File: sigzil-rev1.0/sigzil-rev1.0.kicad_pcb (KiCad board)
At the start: 2 copper layers, 172 x 129.5 mm, 81 parts, among them SW1 Keyswitch, SW10 Keyswitch, SW11 Keyswitch, SW12 Keyswitch, SW13 Keyswitch, SW14 Keyswitch, SW15 Keyswitch, SW16 Keyswitch, SW17 Keyswitch, SW18 Keyswitch, SW19 Keyswitch, SW2 Keyswitch, SW20 Keyswitch, SW21 Keyswitch, SW22 Keyswitch, SW23 Keyswitch, SW24 Keyswitch, SW25 Keyswitch, SW26 Keyswitch, SW27 Keyswitch, SW28 Keyswitch, SW29 Keyswitch, SW3 Keyswitch, SW30 Keyswitch, SW31 Keyswitch, SW32 Keyswitch, SW33 Keyswitch, SW34 Keyswitch, SW35 Keyswitch, SW4 Keyswitch, SW5 Keyswitch, SW6 Keyswitch, SW7 Keyswitch, SW8 Keyswitch, SW9 Keyswitch, U1 Arduino_Pro_Micro

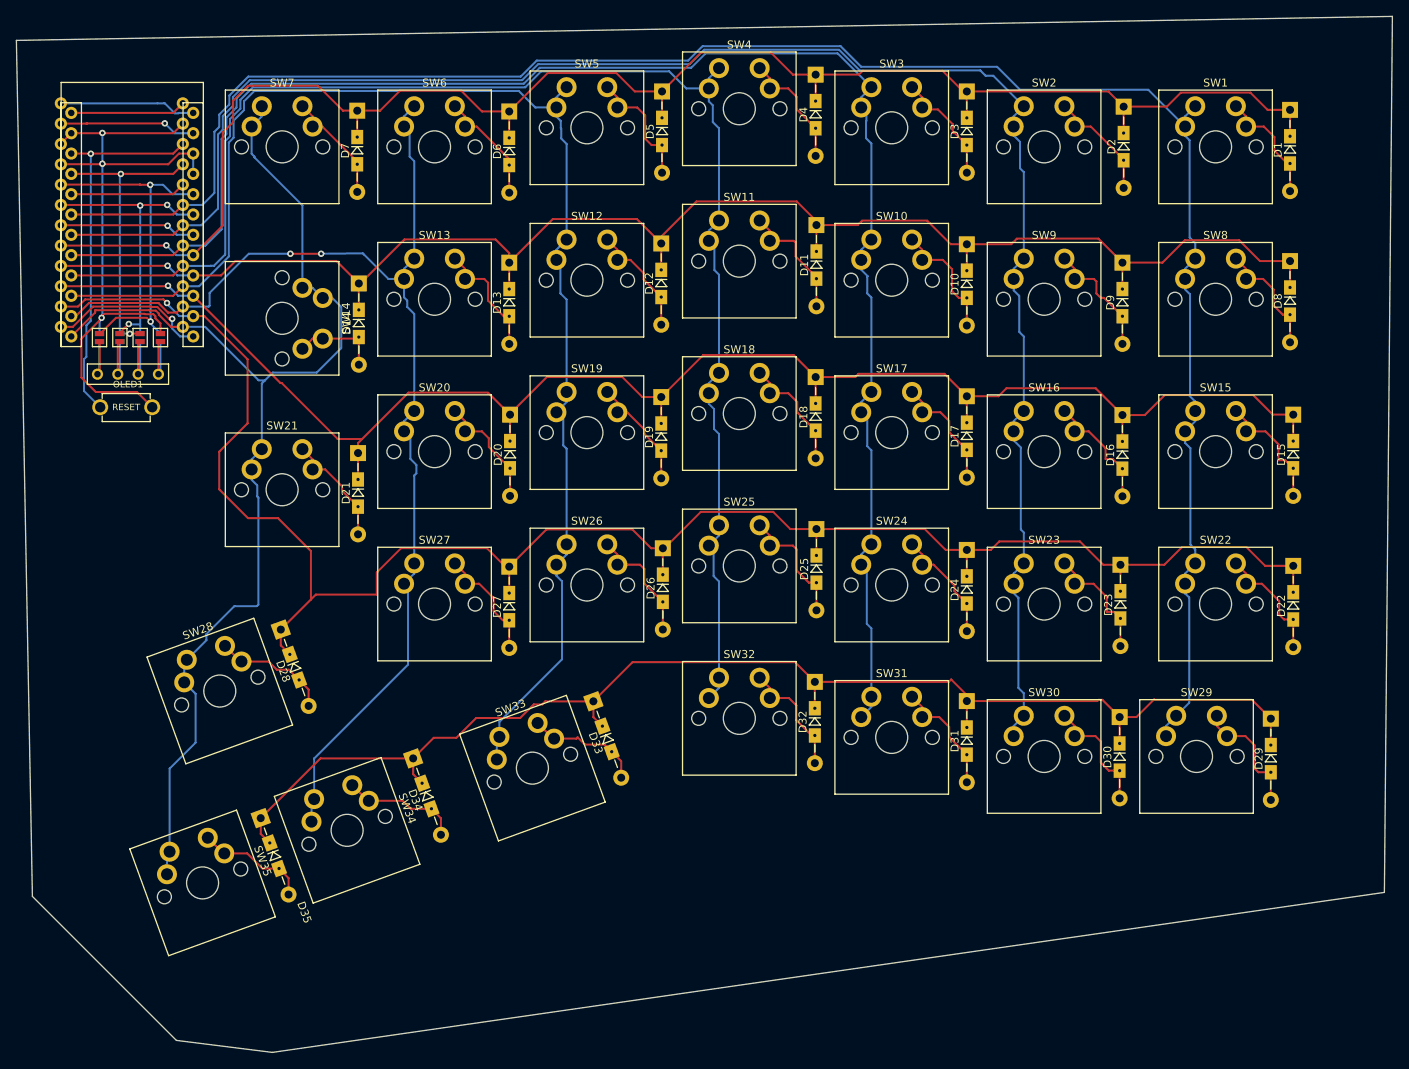
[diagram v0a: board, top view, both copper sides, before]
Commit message: WIP WIP
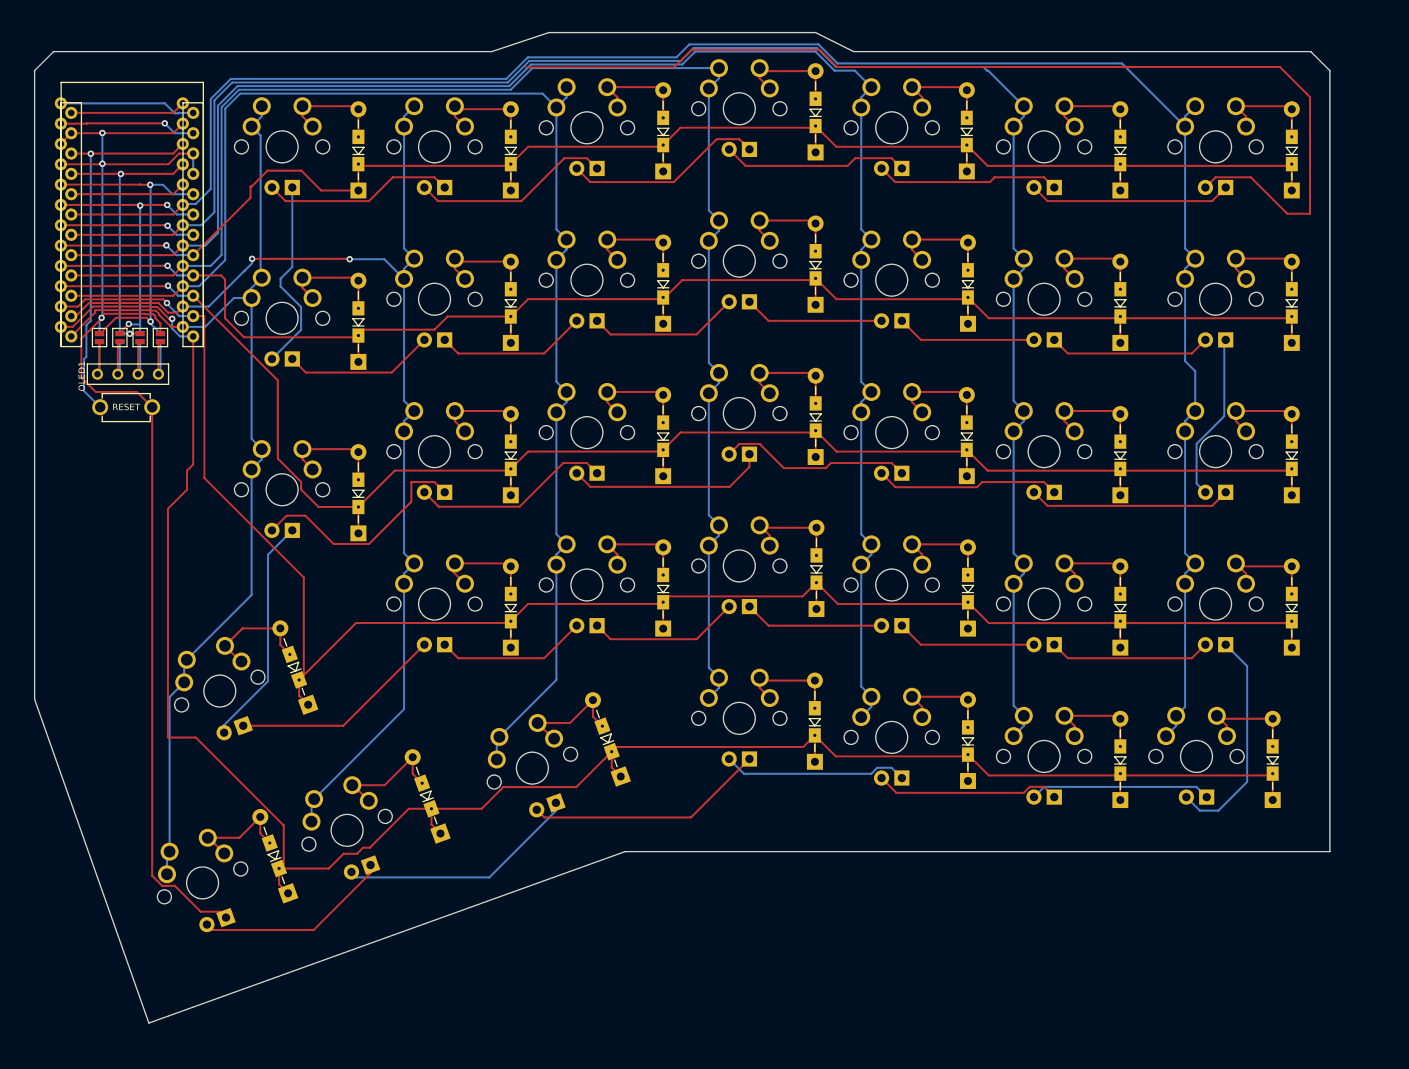
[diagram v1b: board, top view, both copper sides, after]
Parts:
- D1, D10, D11, D12, D13, D14, D15, D16, D17, D18, D19, D2, D20, D21, D22, D23, D24, D25, D26, D27, D28, D29, D3, D30, D31, D32, D33, D34, D35, D4, D5, D6, D7, D8, D9: moved to B.Cu
- SW1, SW15, SW22, SW33, SW8: footprint Sigzil:MX_PCB_1.25u -> Sigzil:MXOnly_Led_1.25u
- SW10, SW11, SW12, SW13, SW16, SW17, SW18, SW19, SW2, SW20, SW21, SW23, SW24, SW25, SW26, SW27, SW28, SW29, SW3, SW30, SW31, SW32, SW4, SW5, SW6, SW7, SW9: footprint Sigzil:MX_PCB_1.00u -> Sigzil:MXOnly_Led_1.00u
- SW14: footprint Sigzil:MX_PCB_1.25u -> Sigzil:MXOnly_Led_1.25u_90deg
- SW34, SW35: footprint Sigzil:MX_PCB_1.25u_90deg -> Sigzil:MXOnly_Led_1.25u_90deg
- moved D2 0.63 mm to (190.3, 54.4), turned to 90 degrees
- moved D30 0.38 mm to (190.3, 130.6), turned to 90 degrees
- moved D23 0.36 mm to (190.3, 111.6), turned to 90 degrees
- moved D8 0.32 mm to (211.8, 73.5), turned to 90 degrees
- moved D29 0.29 mm to (209.4, 130.6), turned to 90 degrees
- moved D22 0.29 mm to (211.8, 111.6), turned to 90 degrees
- moved D4 0.28 mm to (152.2, 49.7), turned to 90 degrees
- moved D19 0.27 mm to (133.2, 90.2), turned to 90 degrees
- moved D9 0.26 mm to (190.3, 73.5), turned to 90 degrees
- moved D16 0.26 mm to (190.3, 92.5), turned to 90 degrees
- moved D12 0.25 mm to (133.2, 71.1), turned to 90 degrees
- moved D27 0.23 mm to (114.1, 111.6), turned to 90 degrees
- moved D1 0.23 mm to (211.8, 54.4), turned to 90 degrees
- moved D6 0.23 mm to (114.1, 54.4), turned to 90 degrees
- moved D24 0.22 mm to (171.3, 109.2), turned to 90 degrees
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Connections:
- U1 pad 7: unconnected-(U1-4/PD4-Pad7) -> BACKLIGHT
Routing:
- net BACKLIGHT: track 0.00 -> 148.6 mm, vias 0 -> 1
- net GND: track 89.8 -> 159.8 mm
- net Row 4: track 184.0 -> 253.5 mm
- net Net-(SW33-Pad): track 0.00 -> 30.3 mm
- net Net-(SW32-Pad): track 0.00 -> 30.0 mm
- net Net-(SW20-Pad): track 0.00 -> 29.0 mm
- net Net-(SW21-Pad): track 0.00 -> 28.8 mm
- net Net-(SW22-Pad): track 0.00 -> 28.1 mm
- net Net-(SW27-Pad): track 0.00 -> 26.8 mm
- net Net-(SW1-Pad): track 0.00 -> 25.4 mm
- net Net-(SW15-Pad): track 0.00 -> 25.4 mm
- net Net-(SW19-Pad): track 0.00 -> 25.1 mm
- net Net-(SW4-Pad): track 0.00 -> 25.0 mm
- net Net-(SW5-Pad): track 0.00 -> 25.0 mm
- net Net-(SW18-Pad): track 0.00 -> 24.9 mm
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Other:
- board size 172 x 129.5 mm -> 161.9 x 123.8 mm
